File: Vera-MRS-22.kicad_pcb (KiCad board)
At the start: 2 copper layers, 58 x 50 mm, 19 parts, among them J4 Screw_Terminal_01x10, Q1 BC337, Q2 BC337, U1 LD1117V50, U2 NUCLEO-F303K8

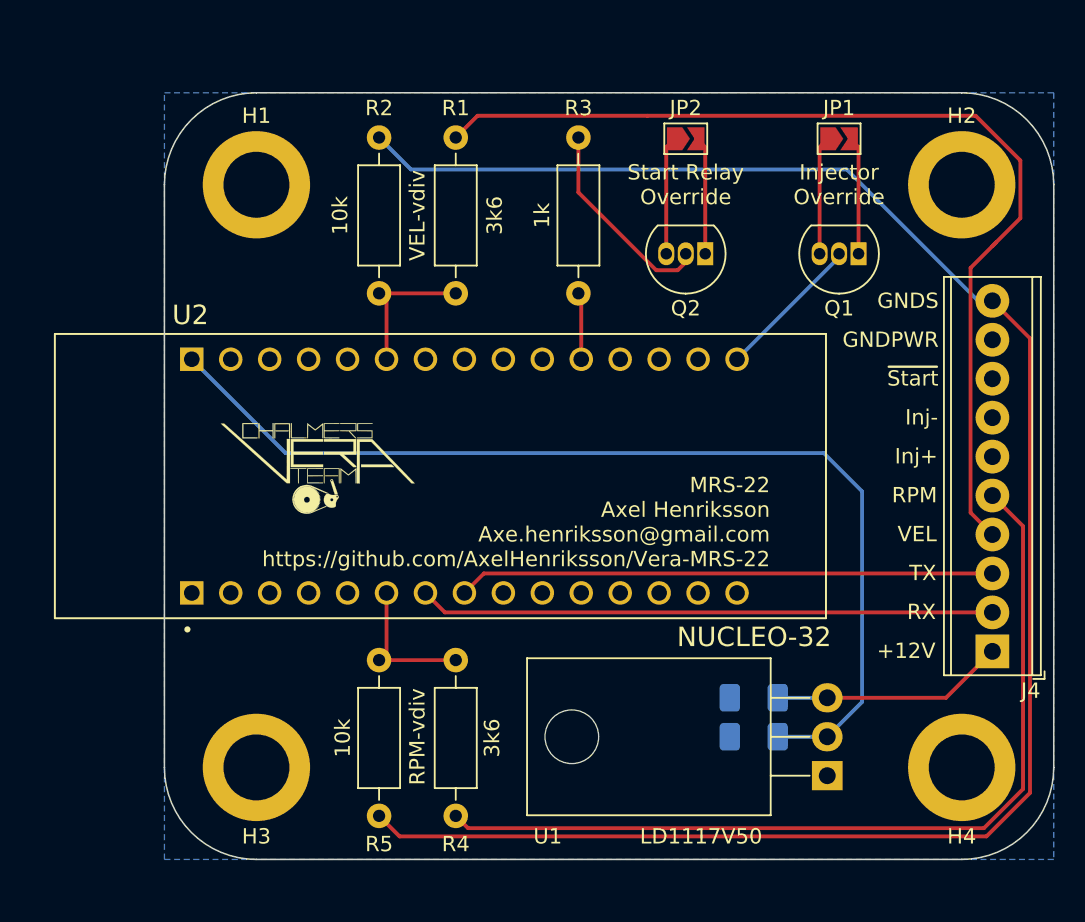
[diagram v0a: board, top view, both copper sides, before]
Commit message: Finished RevB and sent for manufature
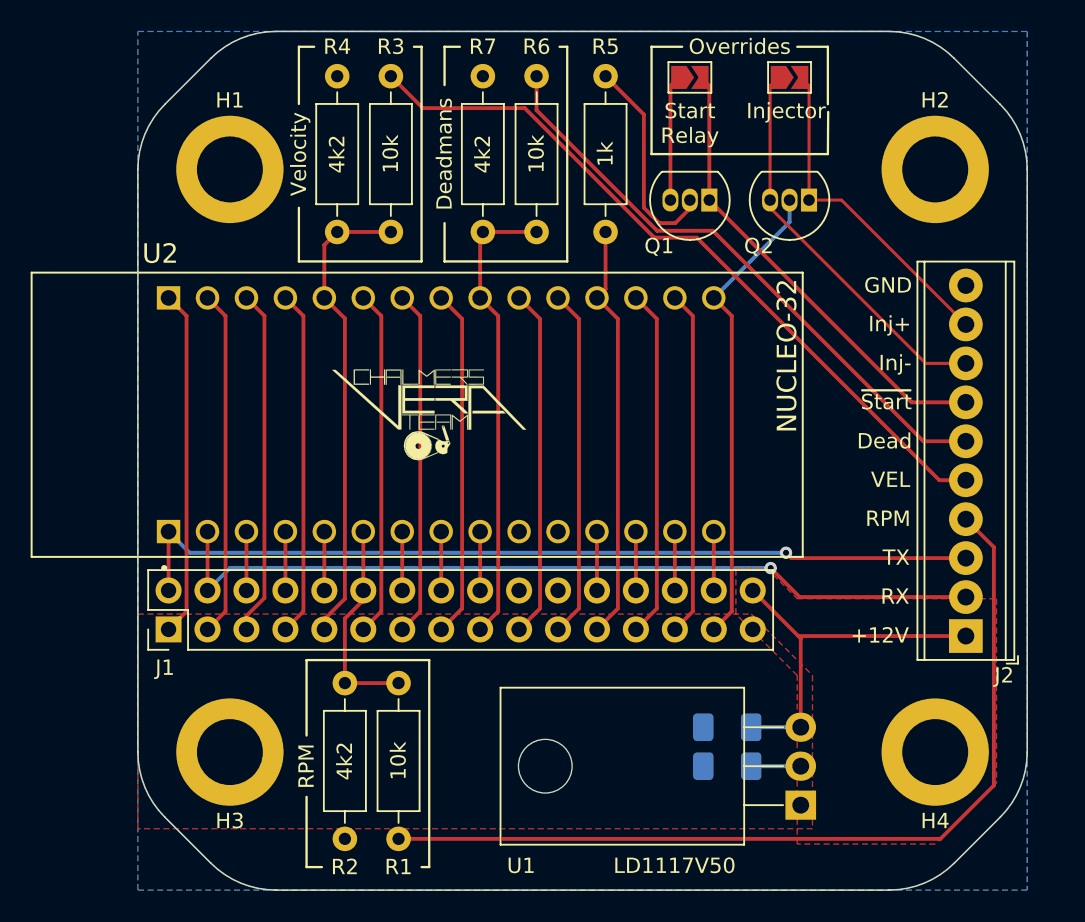
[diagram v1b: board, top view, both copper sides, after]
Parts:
- added J1: 2x16_2.54P_pin_header, Connector_PinHeader_2.54mm:PinHeader_2x16_P2.54mm_Vertical, F.Cu at (175.3, 108.0)
- added R6: 10k, Resistor_THT:R_Axial_DIN0207_L6.3mm_D2.5mm_P10.16mm_Horizontal, F.Cu at (199.3, 71.9)
- added R7: 4k2, Resistor_THT:R_Axial_DIN0207_L6.3mm_D2.5mm_P10.16mm_Horizontal, F.Cu at (195.8, 82.1)
- R1: renamed from R4; value 3k6 -> 10k
- R2: renamed from R5; value 10k -> 4k2
- R3: renamed from R1; value 3k6 -> 10k
- R4: renamed from R2; value 10k -> 4k2
- U2: value NUCLEO-F303K8 -> NUCLEO-G031K8 Physical
- moved G*** 8.07 mm to (192.3, 94.0)
- moved R3 5.82 mm to (189.8, 71.9)
- moved JP2 5.14 mm to (215.8, 72.0)
- moved R4 4.84 mm to (186.3, 82.1)
- moved Q2 4.76 mm to (217.0, 80.0)
- moved R5 4.37 mm to (203.8, 71.9)
- moved U2 4.28 mm to (191.5, 94.0)
- moved R1 4.02 mm to (190.3, 121.7)
- moved JP1 4.01 mm to (209.3, 72.0)
- moved Q1 3.51 mm to (210.5, 80.0)
- moved R2 2.69 mm to (186.8, 111.5)
- moved C1 2.58 mm to (211.7, 114.4)
- moved C2 2.58 mm to (211.7, 116.9)
- moved U1 2.58 mm to (216.5, 119.5)
- moved H1 2.00 mm to (179.3, 78.0)
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- renumbered J4 to J2, JP2 to JP1, JP1 to JP2, Q2 to Q1, Q1 to Q2, R3 to R5
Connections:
- C1 pad 1: GNDPWR -> GND
- C2 pad 1: GNDPWR -> GND
- H1 pad 1: GNDPWR -> GND
- H2 pad 1: GNDPWR -> GND
- H3 pad 1: GNDPWR -> GND
- H4 pad 1: GNDPWR -> GND
- J2 pad 10: GNDS -> GND
- J2 pad 4: /VEL_Tach -> /RPM_Tach
- J2 pad 5: /RPM_Tach -> /VEL_Tach
- J2 pad 6: /Injector_IN -> /Deadmans_12V
- J2 pad 7: /Injector_Out -> /Start_Relay_GND
- J2 pad 8: /Start_Relay_Gnd -> /Injector-
- J2 pad 9: GNDPWR -> /Injector+
- JP1 pad 1: GNDPWR -> GND
- JP2 pad 1: /Injector_OUT -> /Injector-
- JP2 pad 2: /Injector_IN -> /Injector+
- Q1 pad 3: GNDPWR -> GND
- Q2 pad 1: /Injector_IN -> /Injector+
- Q2 pad 3: /Injector_OUT -> /Injector-
- R2 pad 2: GNDS -> GND
- R4 pad 2: GNDS -> GND
- U1 pad 1: GNDPWR -> GND
- U2 pad CN3_1: unconnected-(U2-PadCN3_1) -> /USART1_TX
- U2 pad CN3_10: unconnected-(U2-PadCN3_10) -> Net-(J1-Pad20)
- U2 pad CN3_11: unconnected-(U2-PadCN3_11) -> Net-(J1-Pad22)
- U2 pad CN3_12: unconnected-(U2-PadCN3_12) -> Net-(J1-Pad24)
- U2 pad CN3_13: unconnected-(U2-PadCN3_13) -> Net-(J1-Pad26)
- U2 pad CN3_14: unconnected-(U2-PadCN3_14) -> Net-(J1-Pad28)
- U2 pad CN3_15: unconnected-(U2-PadCN3_15) -> Net-(J1-Pad30)
- U2 pad CN3_2: unconnected-(U2-PadCN3_2) -> /USART1_RX
- U2 pad CN3_3: unconnected-(U2-PadCN3_3) -> Net-(J1-Pad6)
- U2 pad CN3_4: GNDPWR -> GND
- U2 pad CN3_5: unconnected-(U2-PadCN3_5) -> Net-(J1-Pad10)
- U2 pad CN3_7: /USART1_RX -> Net-(J1-Pad14)
- U2 pad CN3_8: /USART1_TX -> Net-(J1-Pad16)
- U2 pad CN3_9: unconnected-(U2-PadCN3_9) -> Net-(J1-Pad18)
- U2 pad CN4_10: unconnected-(U2-PadCN4_10) -> Net-(J1-Pad19)
- U2 pad CN4_11: /Start_Enable -> Net-(J1-Pad21)
- U2 pad CN4_12: unconnected-(U2-PadCN4_12) -> /Start_Enable
- U2 pad CN4_13: unconnected-(U2-PadCN4_13) -> Net-(J1-Pad25)
- U2 pad CN4_14: unconnected-(U2-PadCN4_14) -> Net-(J1-Pad27)
- U2 pad CN4_2: GNDPWR -> GND
- U2 pad CN4_3: unconnected-(U2-PadCN4_3) -> Net-(J1-Pad5)
- U2 pad CN4_4: unconnected-(U2-PadCN4_4) -> Net-(J1-Pad7)
- U2 pad CN4_5: unconnected-(U2-PadCN4_5) -> /VEL
- U2 pad CN4_6: /VEL -> Net-(J1-Pad11)
- U2 pad CN4_7: unconnected-(U2-PadCN4_7) -> Net-(J1-Pad13)
- U2 pad CN4_8: unconnected-(U2-PadCN4_8) -> Net-(J1-Pad15)
- U2 pad CN4_9: unconnected-(U2-PadCN4_9) -> /Deadmans
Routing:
- net GNDS: track 121.7 -> 0.00 mm
- net +5V: track 68.2 -> 25.8 mm
- net /Deadmans_12V: track 0.00 -> 39.2 mm
- net GND: track 0.00 -> 34.7 mm
- net /Deadmans: track 0.00 -> 30.5 mm
- net /Injector-: track 0.00 -> 25.7 mm
- net /Start_Enable: track 4.38 -> 27.3 mm
- net Net-(J1-Pad21): track 0.00 -> 22.8 mm
- net Net-(J1-Pad25): track 0.00 -> 22.8 mm
- net Net-(J1-Pad19): track 0.00 -> 22.8 mm
- net Net-(J1-Pad15): track 0.00 -> 22.8 mm
- net /Start_Relay_GND: track 7.73 -> 30.4 mm
- net Net-(J1-Pad7): track 0.00 -> 22.6 mm
- net Net-(J1-Pad5): track 0.00 -> 22.6 mm
- net Net-(J1-Pad27): track 0.00 -> 22.6 mm
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- added copper zone on F.Cu, net +12V
- added copper zone on F.Cu, net +5V
- added copper zone on B.Cu, net GND
- removed copper zone on B.Cu, net GNDPWR
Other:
- board size 58 x 50 mm -> 58 x 56 mm
- board text added: "Dead"
- board text added: "Deadmans"
- board text added: "GND"
- board text added: "Injector"
- board text added: "JLJLCJLCJLC"
- board text added: "MRS-22 Rev.B Axel Henriksson Axe.henriksson@gmail.com https://github.com/AxelHenriksson/Vera-MRS-22"
- board text added: "Overrides"
- board text added: "Start Relay"
- board text added: "Velocity"
- board text removed: "GNDPWR"
- board text removed: "GNDS"
- board text removed: "Injector Override"
- board text removed: "JLJLCJLC"
- board text removed: "MRS-22 Axel Henriksson Axe.henriksson@gmail.com https://github.com/AxelHenriksson/Vera-MRS-22"
- board text removed: "RPM-vdiv"
- board text removed: "Start Relay Override"
- board text removed: "VEL-vdiv"
